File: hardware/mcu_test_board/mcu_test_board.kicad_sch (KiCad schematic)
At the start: 29 parts, among them CN1 KF2EDGR-2.54-2P, CN2 KF2EDGR-2.54-2P, CN3 SM04B-SRSS-TB (LF)(SN), CN4 KF2EDGR-2.54-4P, J1 Conn_ARM_SWD_TagConnect_TC203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, U1 STM32G474CET6, U2 LD39050PU33R, X1 NX2016SA-16MHZ-EXS00A-CS07826

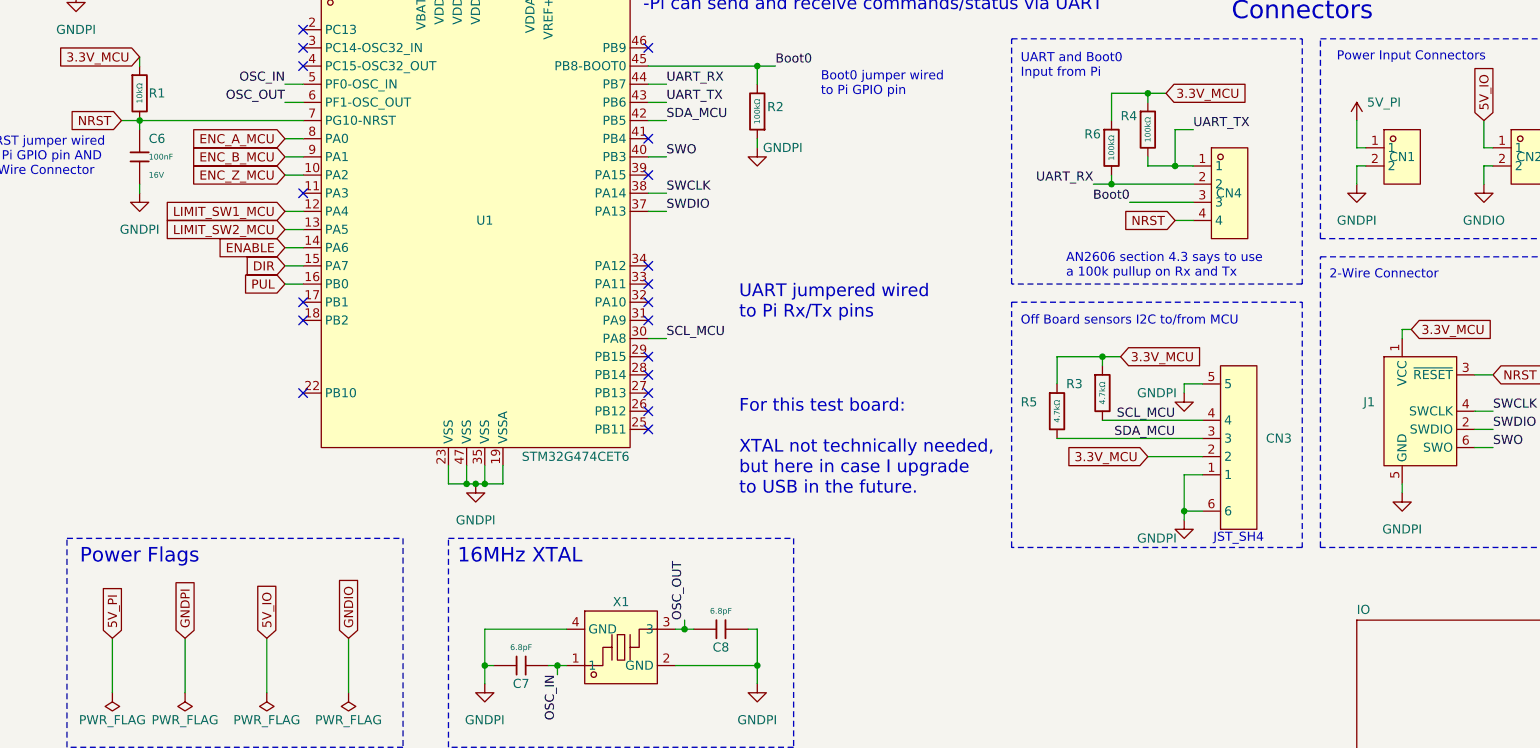
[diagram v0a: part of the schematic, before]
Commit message: Schematic minor improvements - one axis so far
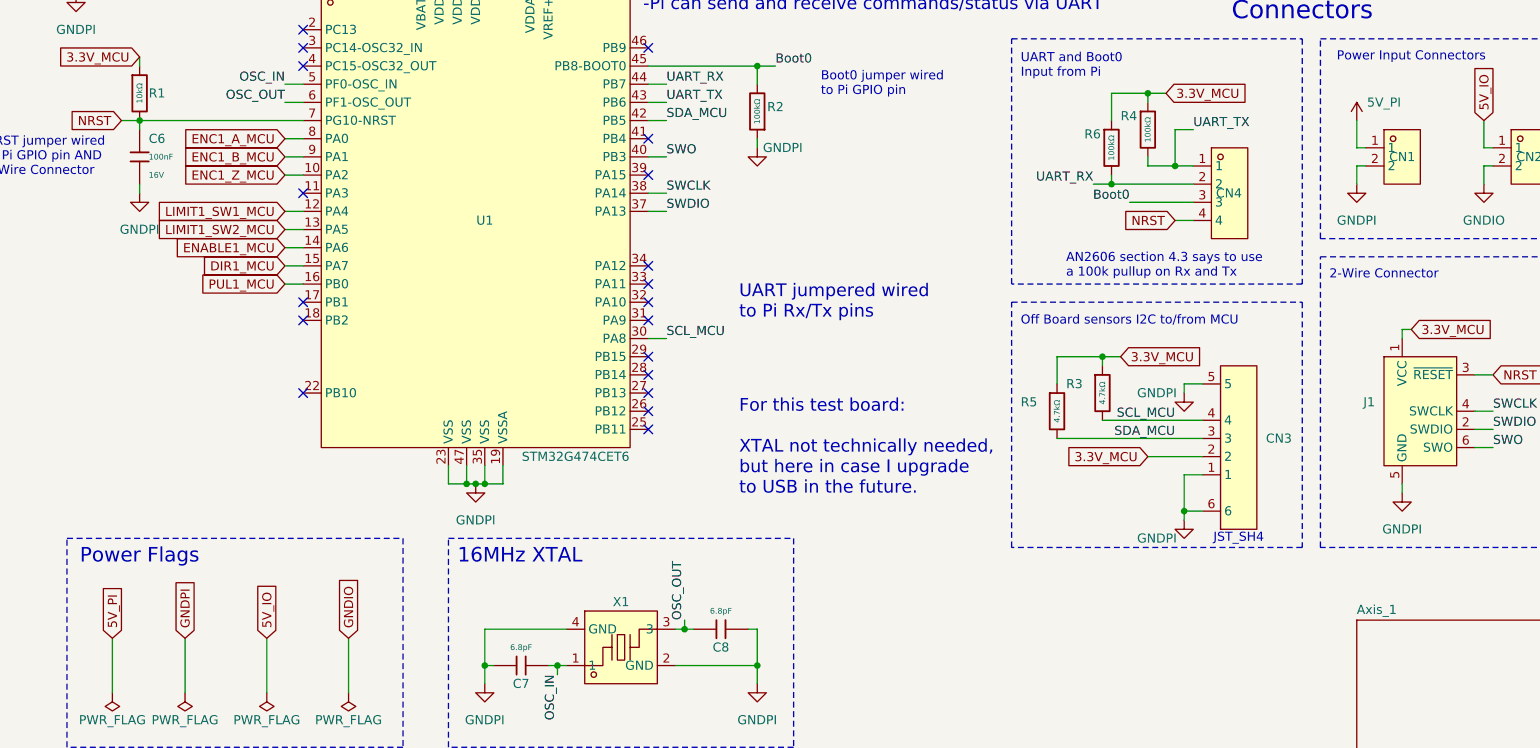
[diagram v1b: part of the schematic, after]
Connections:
- net DIR renamed DIR1_MCU
- net ENABLE renamed ENABLE1_MCU
- net ENC_A_MCU renamed ENC1_A_MCU
- net ENC_B_MCU renamed ENC1_B_MCU
- net ENC_Z_MCU renamed ENC1_Z_MCU
- net LIMIT_SW1_MCU renamed LIMIT1_SW1_MCU
- net LIMIT_SW2_MCU renamed LIMIT1_SW2_MCU
- net PUL renamed PUL1_MCU
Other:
- sheet IO renamed Axis_1
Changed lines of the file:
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@@
 		)
 	)
-	(global_label "ENABLE"
+	(global_label "ENABLE1_MCU"
 		(shape input)
 		(at 55.88 77.47 180)
@@
 		)
 		(property "Intersheetrefs" "${INTERSHEET_REFS}"
-			(at 45.8796 77.47 0)
+			(at 39.6506 77.47 0)
 			(effects
 				(font
@@
 		)
 	)
-	(global_label "PUL"
+	(global_label "PUL1_MCU"
 		(shape input)
 		(at 55.88 82.55 180)
@@
 		)
 		(property "Intersheetrefs" "${INTERSHEET_REFS}"
-			(at 49.2662 82.55 0)
+			(at 43.0372 82.55 0)
 			(effects
 				(font
@@
 		)
 	)
-	(global_label "ENC_Z_MCU"
+	(global_label "ENC1_Z_MCU"
 		(shape input)
 		(at 55.88 67.31 180)
@@
 		)
 		(property "Intersheetrefs" "${INTERSHEET_REFS}"
-			(at 41.9487 67.31 0)
+			(at 40.7392 67.31 0)
 			(effects
 				(font
@@
 		)
 	)
-	(global_label "LIMIT_SW1_MCU"
+	(global_label "LIMIT1_SW1_MCU"
 		(shape input)
 		(at 55.88 72.39 180)
@@
 		)
 		(property "Intersheetrefs" "${INTERSHEET_REFS}"
-			(at 38.3806 72.39 0)
+			(at 37.1711 72.39 0)
 			(effects
 				(font
@@
 		)
 	)
-	(global_label "DIR"
+	(global_label "DIR1_MCU"
 		(shape input)
 		(at 55.88 80.01 180)
@@
 		)
 		(property "Intersheetrefs" "${INTERSHEET_REFS}"
-			(at 49.75 80.01 0)
+			(at 43.521 80.01 0)
 			(effects
 				(font
@@
 		)
 	)
-	(global_label "ENC_A_MCU"
+	(global_label "ENC1_A_MCU"
 		(shape input)
 		(at 55.88 62.23 180)
@@
 		)
 		(property "Intersheetrefs" "${INTERSHEET_REFS}"
-			(at 42.0696 62.23 0)
+			(at 40.8601 62.23 0)
 			(effects
 				(font
@@
 		)
 	)
-	(global_label "ENC_B_MCU"
+	(global_label "ENC1_B_MCU"
 		(shape input)
 		(at 55.88 64.77 180)
@@
 		)
 		(property "Intersheetrefs" "${INTERSHEET_REFS}"
-			(at 41.8882 64.77 0)
+			(at 40.6787 64.77 0)
 			(effects
 				(font
@@
 		)
 	)
-	(global_label "LIMIT_SW2_MCU"
+	(global_label "LIMIT1_SW2_MCU"
 		(shape input)
 		(at 55.88 74.93 180)
@@
 		)
 		(property "Intersheetrefs" "${INTERSHEET_REFS}"
-			(at 38.3806 74.93 0)
+			(at 37.1711 74.93 0)
 			(effects
 				(font
@@
 			(color 0 0 0 0.0000)
 		)
-		(property "Sheetname" "IO"
+		(property "Sheetname" "Axis_1"
 			(at 205.74 128.8284 0)
 			(effects
